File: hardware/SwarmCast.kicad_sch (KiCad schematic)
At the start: 0 parts

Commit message: PCB design completed
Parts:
- added C1, C10, C11, C12, C13, C2, C3, C4, C5, C6, C7, C8, C9: 0.1u, Capacitor_THT:C_Disc_D5.0mm_W2.5mm_P2.50mm, symbol Device:C_Small
- added H1, H2, H3, H4: MountingHole, MountingHole:MountingHole_3.2mm_M3, symbol Mechanical:MountingHole
- added J1: POWER-IN, Connector_JST:JST_XH_B2B-XH-A_1x02_P2.50mm_Vertical, symbol Connector_Generic:Conn_01x02
- added J2: LDR, Connector_JST:JST_XH_B2B-XH-A_1x02_P2.50mm_Vertical, symbol Connector_Generic:Conn_01x02
- added JP1, JP2, JP3, JP4: SJ, Jumper:SolderJumper-3_P1.3mm_Open_RoundedPad1.0x1.5mm, symbol Jumper:SolderJumper_3_Open
- added Q1, Q2, Q3, Q4: BC547_npn, pcbcupid_footprint:BC547_npn, symbol pcbcupid:BC547_npn
- added R1, R11, R12, R13, R17, R18, R19, R2, R3, R4, R5, R6, R7, R8: 100, Resistor_THT:R_Axial_DIN0207_L6.3mm_D2.5mm_P7.62mm_Horizontal, symbol Device:R_Small
- added R10, R15, R16, R20, R9: 4k7, Resistor_THT:R_Axial_DIN0207_L6.3mm_D2.5mm_P7.62mm_Horizontal, symbol Device:R_Small
- added R14: 10k, Resistor_THT:R_Axial_DIN0207_L6.3mm_D2.5mm_P7.62mm_Horizontal, symbol Device:R_Small
- added SW1: SW_Push, Button_Switch_THT:SW_PUSH-12mm, symbol Switch:SW_Push
- added SW2, SW3: SW_Push, Button_Switch_THT:SW_PUSH_6mm_H5mm, symbol Switch:SW_Push
- added U1: glyph-s3, pcbcupid_footprint:glyph-s3, symbol pcbcupid:glyph-s3
- added U2: DHT 11, pcbcupid_footprint:DHT11, symbol pcbcupid:DHT 11
- added U3: gmod-micro_sd, pcbcupid_footprint:gmod-micro_sd, symbol pcbcupid:gmod-micro_sd
- added U4: gmod-rtc, pcbcupid_footprint:gmod-rtc, symbol pcbcupid:gmod-rtc
- added U5, U6, U7, U8: gsense-microphone_1ch, pcbcupid_footprint:gsense-microphone_1ch, symbol pcbcupid:gsense-microphone_1ch
- added U9: OLED 0.91 DISPLAY, pcbcupid_footprint:OLED_0.91_display, symbol pcbcupid:oled_0.91_display
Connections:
- new net: JP3.2 (C), U5.2 (LR)
- new net: Q4.2 (BASE), R7.2, R8.2
- new net: R13.1, SW3.2
- new net: Q4.1 (COLLECTOR), U5.1 (GND)
- new net: R12.1, SW2.2
- new net: Q3.2 (BASE), R5.2, R6.2
- new net: JP4.2 (C), U7.2 (LR)
- new net: Q3.1 (COLLECTOR), U7.1 (GND)
- new net: JP1.2 (C), U8.2 (LR)
- new net: Q1.2 (BASE), R1.2, R2.2
- new net: Q2.2 (BASE), R3.2, R4.2
- new net: R11.1, SW1.2
- new net: Q2.1 (COLLECTOR), U8.1 (GND)
- new net: Q1.1 (COLLECTOR), U6.1 (GND)
- new net: JP2.2 (C), U6.2 (LR)
- new net +3.3V: C10.1, C11.1, C4.1, C5.1, C6.1, C7.1, C8.1, C9.1, J2.2 (Pin_2), JP1.1 (A), JP2.1 (A), JP3.1 (A), JP4.1 (A), R10.2, R15.2, R16.2, R17.2, R18.2, R19.2, R20.2, R9.2, U1.14 (3V3), U1.15 (3V3), U2.1 (VDD), U3.9 (3V3), U4.6 (VCC), U5.6 (VCC), U6.6 (VCC), U7.6 (VCC), U8.6 (VCC), U9.2 (VCC_IN)
- new net BT1: C1.1, R11.2, R17.1, U1.27 (TX)
- new net BT2: C2.1, R12.2, R18.1, U1.17 (D13)
- new net BT3: C3.1, R13.2, R19.1, U1.26 (RX)
- new net CS: R15.1, U1.22 (D18), U3.4 (CS)
- new net DATA: R20.1, U1.21 (D17), U2.2 (DATA)
- new net GND: C1.2, C10.2, C11.2, C12.2, C13.2, C2.2, C3.2, C4.2, C5.2, C6.2, C7.2, C8.2, C9.2, J1.1 (Pin_1), JP1.3 (B), JP2.3 (B), JP3.3 (B), JP4.3 (B), Q1.3 (EMITTER), Q2.3 (EMITTER), Q3.3 (EMITTER), Q4.3 (EMITTER), R14.1, R2.1, R4.1, R6.1, R8.1, SW1.1, SW2.1, SW3.1, U1.16 (GND), U1.28 (GND), U2.4 (GND), U3.2 (GND), U4.5 (GND), U9.1 (GND)
- new net LDR: J2.1 (Pin_1), R14.2, U1.4 (A2)
- new net MI: R16.1, U1.25 (MI), U3.5 (MI)
- new net MIC1: R1.1, R5.1, U1.8 (A9)
- new net MIC2: R3.1, R7.1, U1.9 (A10)
- new net MO: U1.24 (MO), U3.6 (MO)
- new net SCK: U1.23 (SCK), U3.7 (SCK)
- new net SCK_M1: U1.20 (D16), U6.5 (SCK), U8.5 (SCK)
- new net SCK_M2: U1.5 (A6), U5.5 (SCK), U7.5 (SCK)
- new net SCL: R9.1, U1.1 (SCL), U4.1 (SCL), U9.3 (SCL)
- new net SDA: R10.1, U1.2 (SDA), U4.2 (SDA), U9.4 (SDA)
- new net SD_M1: U1.19 (D15), U6.4 (SD), U8.4 (SD)
- new net SD_M2: U1.6 (A7), U5.4 (SD), U7.4 (SD)
- new net VCC: C12.1, C13.1, J1.2 (Pin_2), U1.12 (BAT)
- new net WS_M1: U1.18 (D14), U6.3 (WS), U8.3 (WS)
- new net WS_M2: U1.7 (A8), U5.3 (WS), U7.3 (WS)
- no-connect marks 0 -> 8

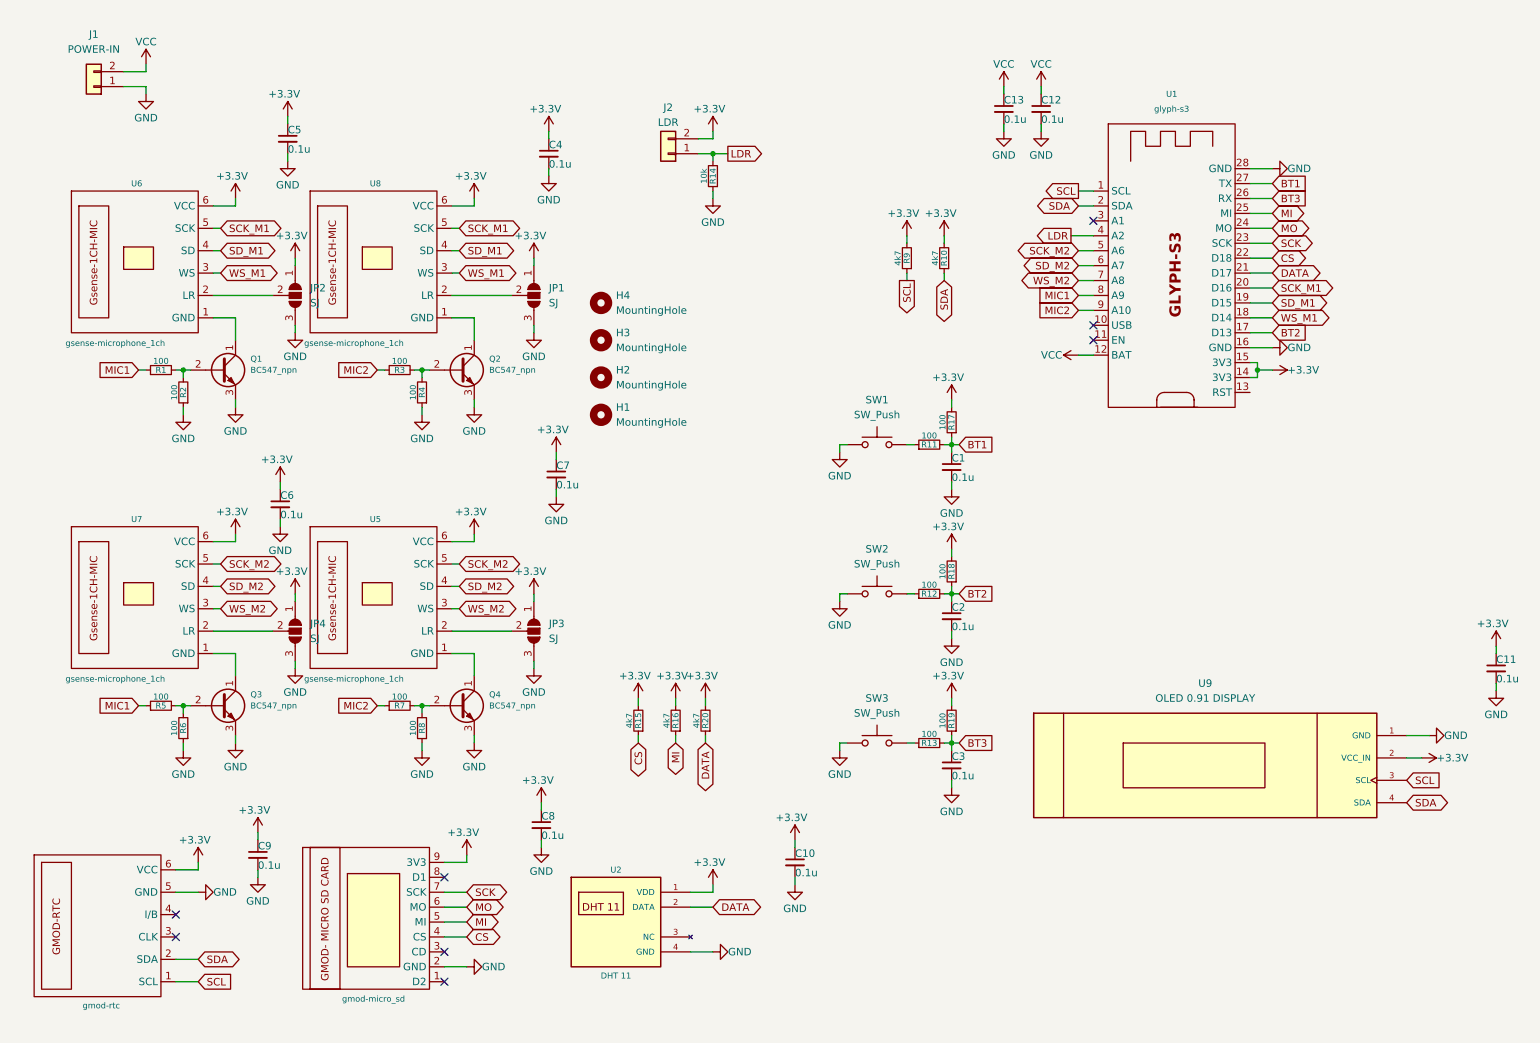
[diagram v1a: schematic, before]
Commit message: Update: PCB files
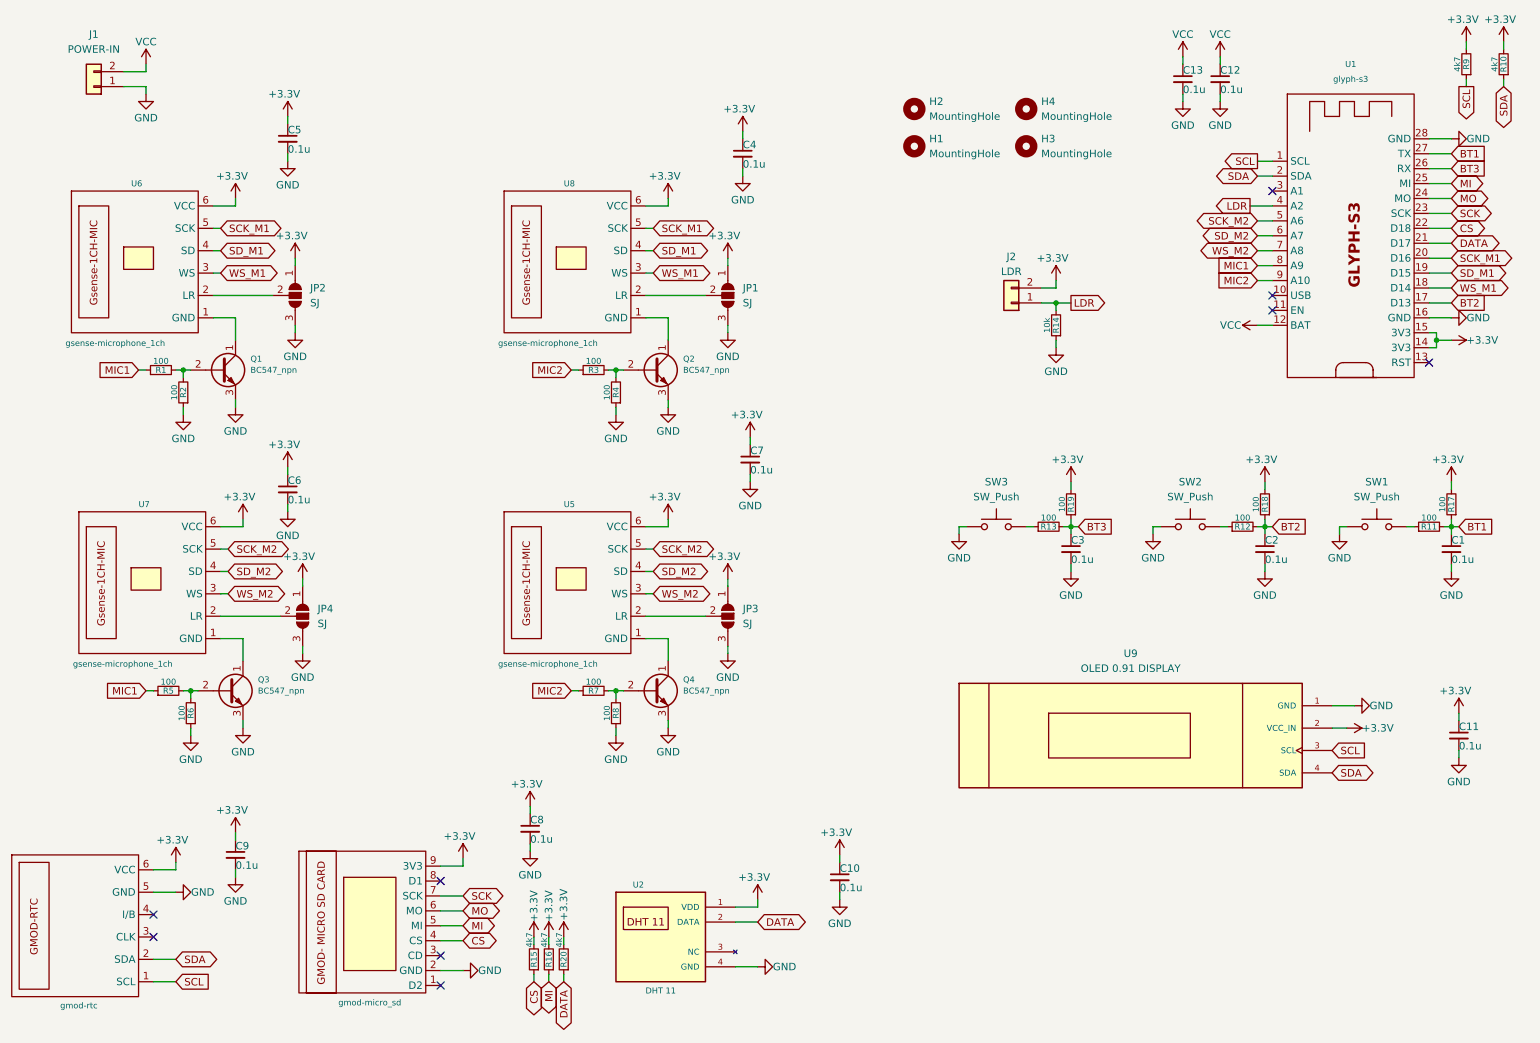
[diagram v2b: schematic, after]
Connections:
- no-connect marks 8 -> 9
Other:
- moved on the sheet: C1, C10, C11, C12, C13, C2, C3, C4, C6, C7, C8, C9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
